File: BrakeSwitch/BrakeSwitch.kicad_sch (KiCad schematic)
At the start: 16 parts, among them J1 12V_in, J2 LightPlug, J3 5V_out, J4 Front_Loop, J5 Rear_Loop, J6 12V_Out, Q1 NMOS, U2 LMV321, U3 LMV321

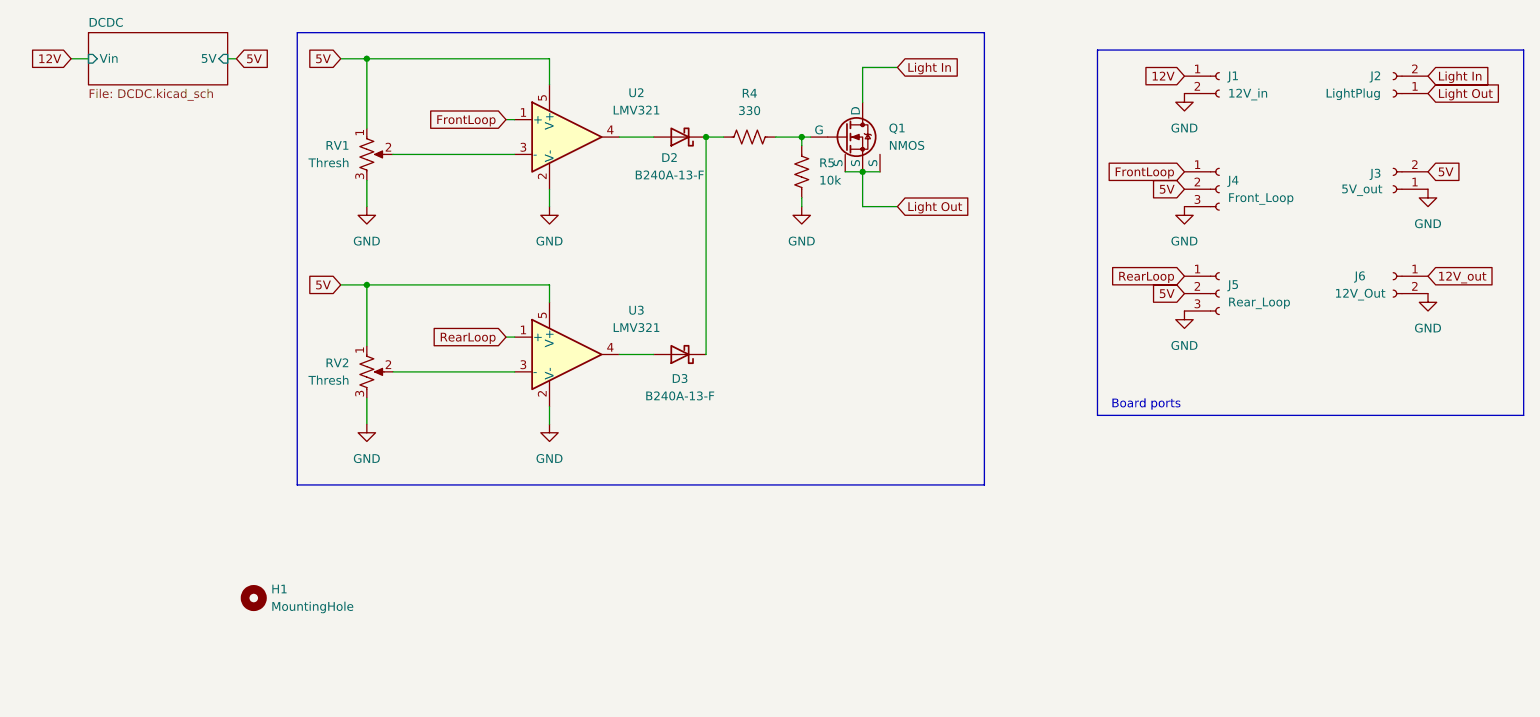
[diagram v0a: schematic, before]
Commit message: Progress save
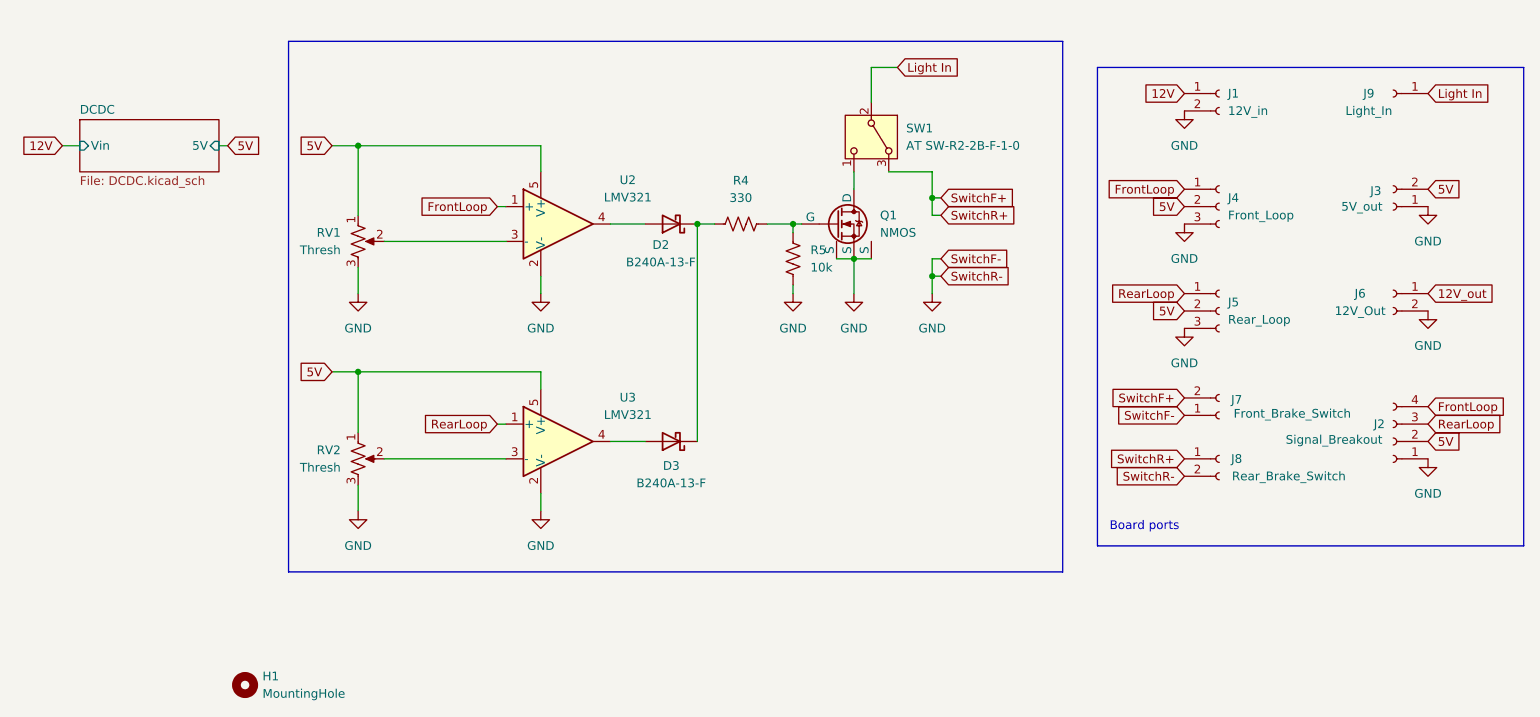
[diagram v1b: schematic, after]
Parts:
- removed J2: LightPlug, AA-Custom:SolderPad_01x02, symbol Connector:Conn_01x02_Socket
- added J2: Signal_Breakout, AA-Custom:SolderPad_01x04, symbol Connector:Conn_01x04_Socket
- added J7: Front_Brake_Switch, AA-Custom:SolderPad_01x02, symbol Connector:Conn_01x02_Socket
- added J8: Rear_Brake_Switch, AA-Custom:SolderPad_01x02, symbol Connector:Conn_01x02_Socket
- added J9: Light_In, AA-Custom:SolderPad_01x01, symbol Connector:Conn_01x01_Socket
- added SW1: AT SW-R2-2B-F-1-0, AA-Custom:SPDT_PanelMount_Switch, symbol Switch:SW_Nidec_CAS-120A1
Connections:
- net Light Out is gone; now on net GND: Q1.1 (S), Q1.2 (S), Q1.3 (S)
- net 5V: now also J2.2 (Pin_2)
- net FrontLoop: now also J2.4 (Pin_4)
- net GND: now also J2.1 (Pin_1), J7.1 (Pin_1), J8.2 (Pin_2)
- net Light In: now also J9.1 (Pin_1), SW1.2 (B); no longer Q1.5 (D)
- net RearLoop: now also J2.3 (Pin_3)
- new net: Q1.5 (D), SW1.1 (C)
- new net SwitchF+: J7.2 (Pin_2), J8.1 (Pin_1), SW1.3 (A)
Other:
- moved on the sheet: D2, D3, H1, J1, J3, J4, J5, J6, Q1, R4, R5, RV1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

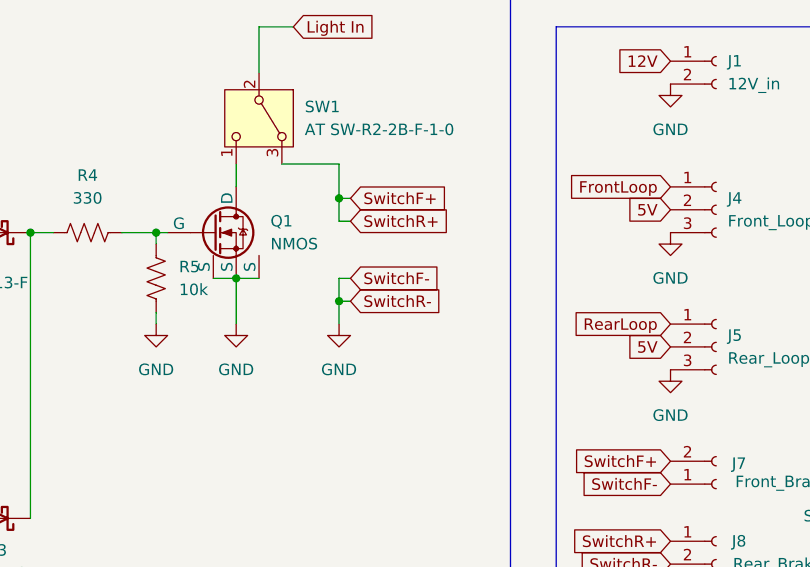
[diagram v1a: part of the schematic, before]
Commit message: Layout doneish
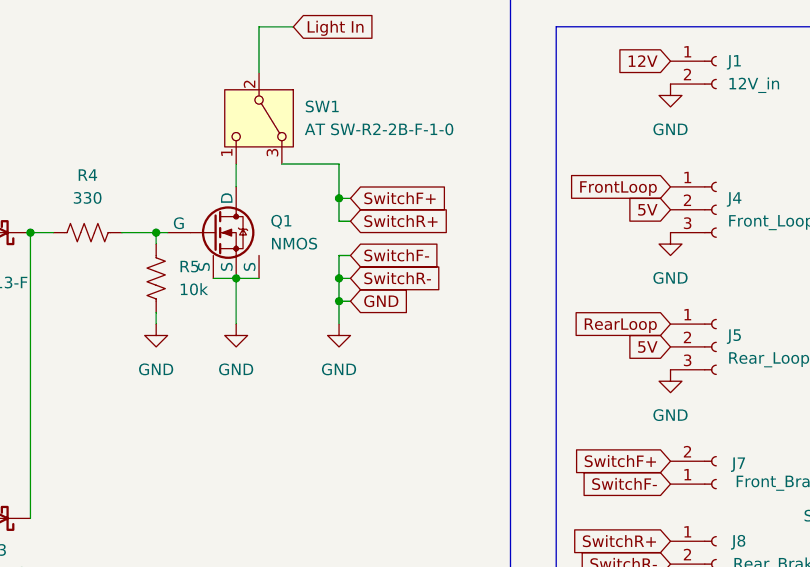
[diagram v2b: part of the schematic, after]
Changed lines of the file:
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@@
+	)
+	(junction
+		(at 147.32 53.34)
+		(diameter 0)
+		(color 0 0 0 0)
+	)
+	(junction
+		(at 127 48.26)
+		(diameter 0)
+		(color 0 0 0 0)
 	)
 	(junction
@@
 		(color 0 0 0 0)
 	)
-	(junction
-		(at 127 48.26)
-		(diameter 0)
-		(color 0 0 0 0)
-	)
 	(wire
 		(pts
@@
 	(wire
 		(pts
+			(xy 147.32 53.34) (xy 148.59 53.34)
+		)
+		(stroke
+			(width 0)
+			(type default)
+		)
+	)
+	(wire
+		(pts
 			(xy 147.32 55.88) (xy 148.59 55.88)
 		)
@@
 	(wire
 		(pts
+			(xy 147.32 53.34) (xy 147.32 50.8)
+		)
+		(stroke
+			(width 0)
+			(type default)
+		)
+	)
+	(wire
+		(pts
 			(xy 90.17 36.83) (xy 90.17 40.64)
 		)
@@
 	(wire
 		(pts
+			(xy 147.32 55.88) (xy 147.32 58.42)
+		)
+		(stroke
+			(width 0)
+			(type default)
+		)
+	)
+	(wire
+		(pts
 			(xy 83.82 45.72) (xy 85.09 45.72)
 		)
@@
 	(wire
 		(pts
-			(xy 147.32 53.34) (xy 148.59 53.34)
+			(xy 147.32 50.8) (xy 148.59 50.8)
 		)
 		(stroke
@@
 	(wire
 		(pts
-			(xy 147.32 58.42) (xy 147.32 55.88)
-		)
-		(stroke
-			(width 0)
-			(type default)
-		)
-	)
-	(wire
-		(pts
 			(xy 148.59 46.99) (xy 147.32 46.99)
 		)
@@
 	(wire
 		(pts
-			(xy 147.32 55.88) (xy 147.32 53.34)
+			(xy 147.32 53.34) (xy 147.32 55.88)
 		)
 		(stroke
@@
 		)
 	)
+	(global_label "GND"
+		(shape input)
+		(at 148.59 55.88 0)
+		(fields_autoplaced yes)
+		(effects
+			(font
+				(size 1.27 1.27)
+			)
+			(justify left)
+		)
+		(property "Intersheetrefs" "${INTERSHEET_REFS}"
+			(at 155.4457 55.88 0)
+			(effects
+				(font
+					(size 1.27 1.27)
+				)
+				(justify left)
+				(hide yes)
+			)
+		)
+	)
 	(global_label "5V"
 		(shape input)
@@
 	(global_label "SwitchR-"
 		(shape input)
-		(at 148.59 55.88 0)
-		(fields_autoplaced yes)
-		(effects
-			(font
-				(size 1.27 1.27)
-			)
-			(justify left)
-		)
-		(property "Intersheetrefs" "${INTERSHEET_REFS}"
-			(at 160.5257 55.88 0)
+		(at 148.59 53.34 0)
+		(fields_autoplaced yes)
+		(effects
+			(font
+				(size 1.27 1.27)
+			)
+			(justify left)
+		)
+		(property "Intersheetrefs" "${INTERSHEET_REFS}"
+			(at 160.5257 53.34 0)
 			(effects
 				(font
@@
 	(global_label "SwitchF-"
 		(shape input)
-		(at 148.59 53.34 0)
-		(fields_autoplaced yes)
-		(effects
-			(font
-				(size 1.27 1.27)
-			)
-			(justify left)
-		)
-		(property "Intersheetrefs" "${INTERSHEET_REFS}"
-			(at 160.3443 53.34 0)
-			(effects
-				(font
+		(at 148.59 50.8 0)
+		(fields_autoplaced yes)
+		(effects
+			(font
+				(size 1.27 1.27)
+			)
+			(justify left)
+		)
+		(property "Intersheetrefs" "${INTERSHEET_REFS}"
+			(at 160.3443 50.8 0)
+			(effects
+				(font
